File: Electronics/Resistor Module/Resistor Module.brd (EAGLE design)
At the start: 50 x 50 mm, 121 parts, among them U1 74HC595D, U2 74HC595D, U3 74HC595D, U4 74HC595D, U5 25AA010A

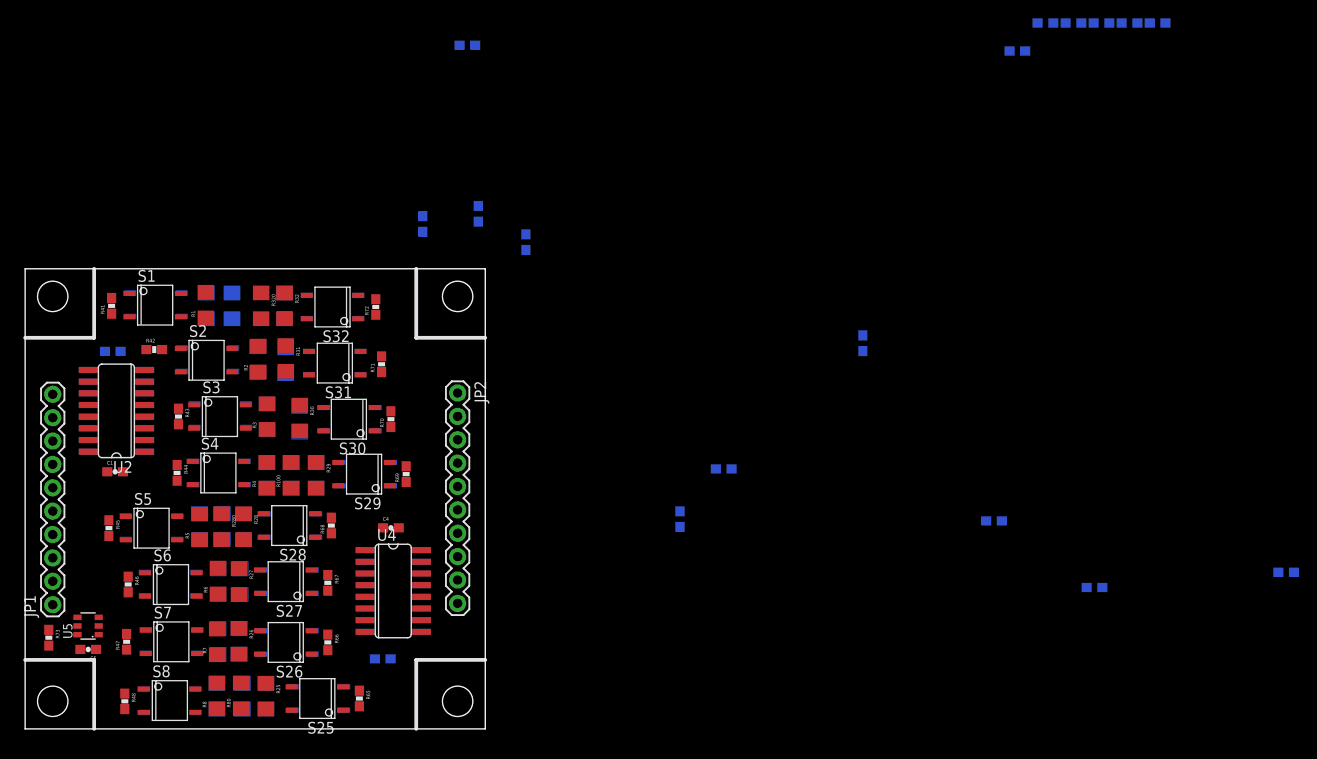
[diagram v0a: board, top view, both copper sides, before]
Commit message: Everything in it's place
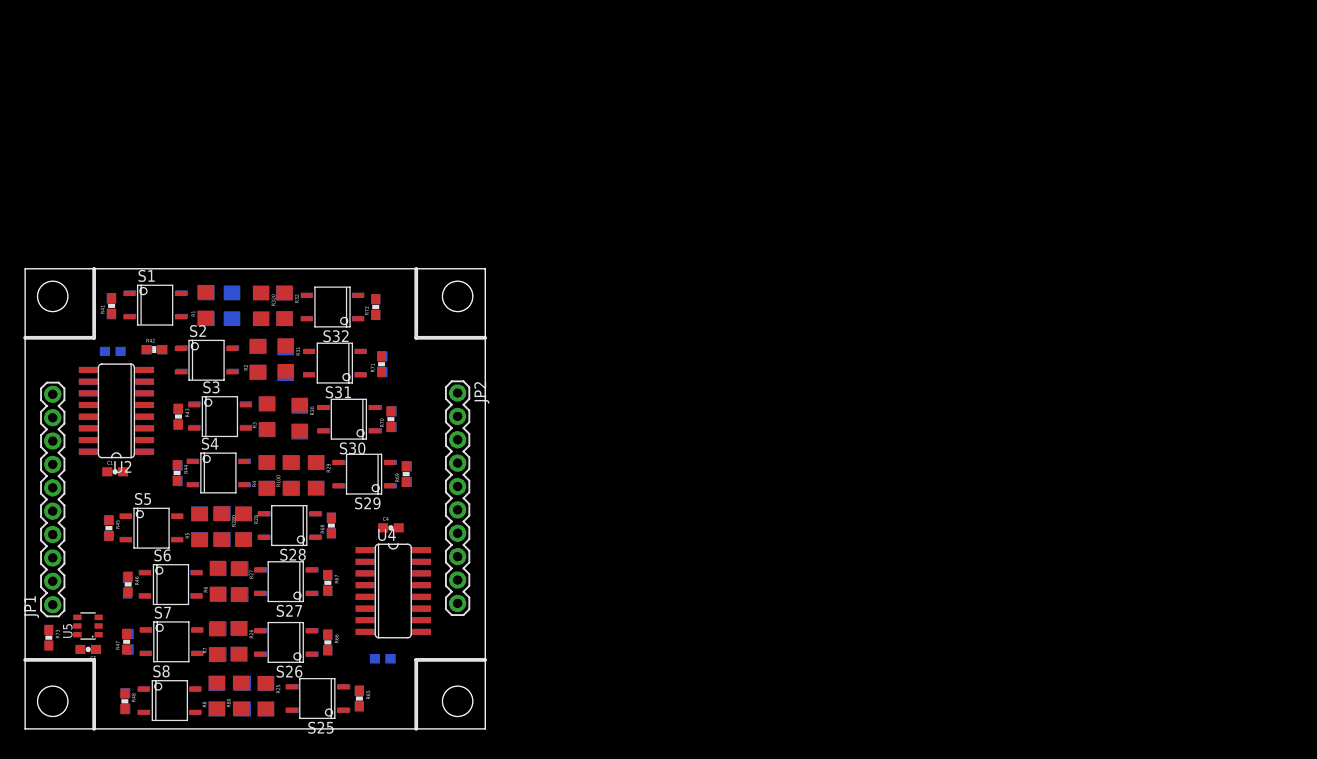
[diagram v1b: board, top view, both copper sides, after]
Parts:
- moved R49 126.9 mm to (10.9, 3.05), turned to 270 degrees
- moved R63 103.0 mm to (32.9, 9.40), turned to 270 degrees
- moved R62 101.3 mm to (32.9, 15.9), turned to 90 degrees
- moved R61 99.9 mm to (33.3, 22.1), turned to 90 degrees
- moved R59 93.7 mm to (39.9, 33.7), turned to 90 degrees
- moved R60 92.5 mm to (41.5, 27.7), turned to 90 degrees
- moved R64 80.8 mm to (36.3, 3.30), turned to 270 degrees
- moved R58 76.9 mm to (38.9, 39.6), turned to 90 degrees
- moved R54 74.9 mm to (16.6, 33.9)
- moved R50 74.5 mm to (11.3, 9.47), turned to 270 degrees
- moved R57 71.1 mm to (38.1, 45.8), turned to 90 degrees
- moved R56 66.0 mm to (9.36, 45.9), turned to 90 degrees
- moved R55 63.2 mm to (14.1, 41.2)
- moved R51 57.2 mm to (11.1, 15.6), turned to 270 degrees
- moved R52 47.5 mm to (9.12, 21.8), turned to 270 degrees
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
